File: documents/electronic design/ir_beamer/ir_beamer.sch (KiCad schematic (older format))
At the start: 10 parts, among them P1 STM32F103_header, U1 74HC595D

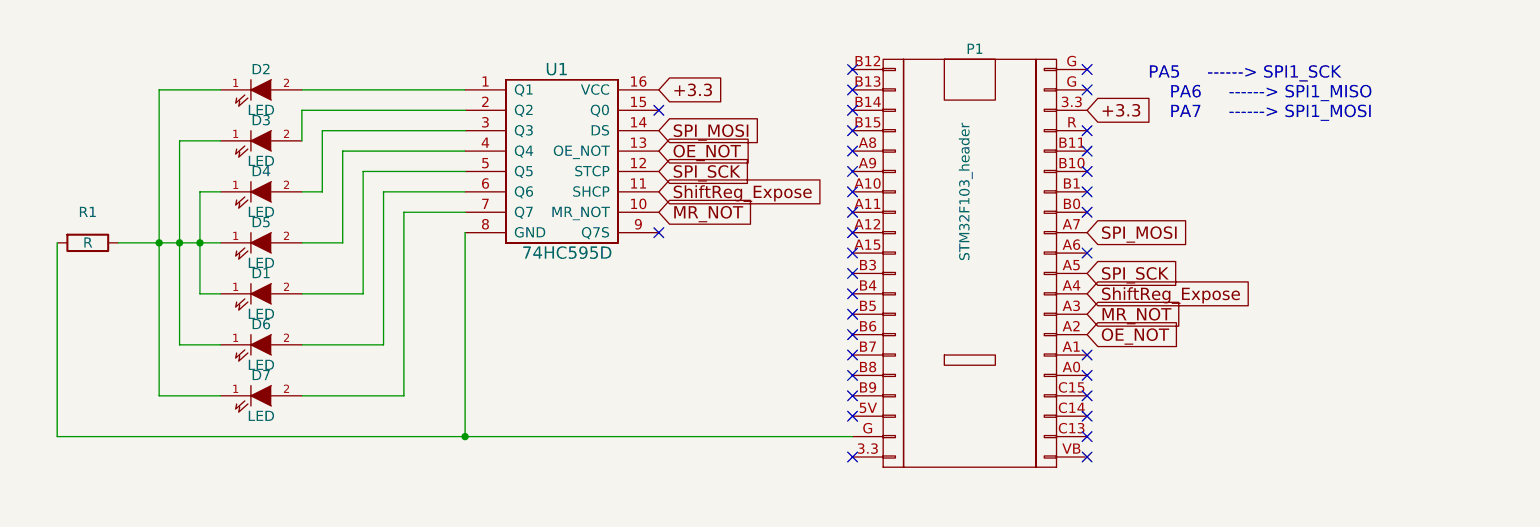
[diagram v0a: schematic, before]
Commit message: update pcb
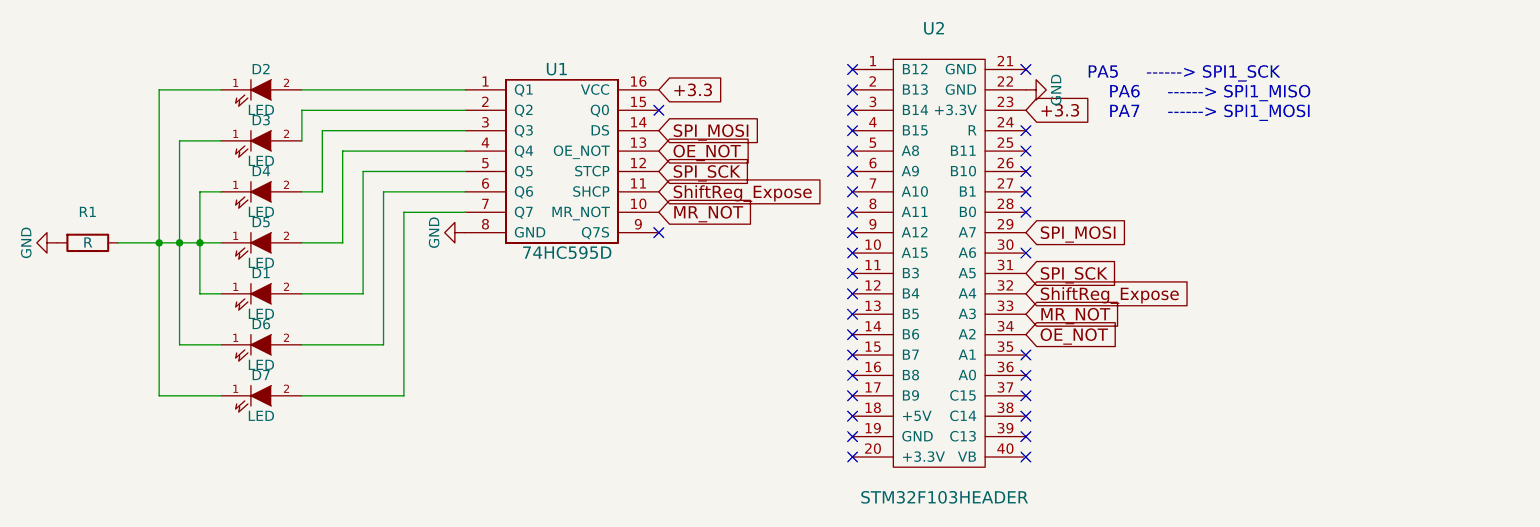
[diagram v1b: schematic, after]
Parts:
- removed P1: STM32F103_header, footprints:STM32F103C8T6_pin_header, symbol STM32F103_header
- added U2: STM32F103HEADER, symbol STM32F103HEADER
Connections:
- net +3.3: now also U2.23 (+3.3V)
- net MR_NOT: now also U2.33 (A3)
- net OE_NOT: now also U2.34 (A2)
- net SPI_MOSI: now also U2.29 (A7)
- net SPI_SCK: now also U2.31 (A5)
- net ShiftReg_Expose: now also U2.32 (A4)
- net GND: now reaches R1.2, U1.8 (GND)
- net GND: now also U2.22 (GND)
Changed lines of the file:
@@
 NoConn ~ 5300 3050
 NoConn ~ 5300 3150
-NoConn ~ 6450 3350
-NoConn ~ 6450 3250
-NoConn ~ 6450 3150
-NoConn ~ 6450 3050
-NoConn ~ 6450 2950
-NoConn ~ 6450 2850
-NoConn ~ 6450 2150
-NoConn ~ 6450 1950
-NoConn ~ 6450 1850
-NoConn ~ 6450 1750
+NoConn ~ 6150 3350
+NoConn ~ 6150 3250
+NoConn ~ 6150 3150
+NoConn ~ 6150 3050
+NoConn ~ 6150 2950
+NoConn ~ 6150 2850
+NoConn ~ 6150 2150
+NoConn ~ 6150 1950
+NoConn ~ 6150 1850
+NoConn ~ 6150 1750
 $Comp
 L LED D1
@@
 	1    0    0    -1
 $EndComp
-$Comp
-L STM32F103_header P1
-U 1 1 578765C4
-P 5500 2400
-F 0 "P1" H 5900 3450 50  0000 C CNN
-F 1 "STM32F103_header" V 5850 2750 50  0000 C CNN
-F 2 "footprints:STM32F103C8T6_pin_header" H 5500 2400 50  0001 C CNN
-F 3 "" H 5500 2400 50  0000 C CNN
-	1    5500 2400
-	1    0    0    -1
-$EndComp
-Text Notes 6750 1700 0    60   ~ 0
+Text Notes 6450 1700 0    60   ~ 0
     PA5     ------> SPI1_SCK\n    PA6     ------> SPI1_MISO\n    PA7     ------> SPI1_MOSI
-Text GLabel 6450 2450 2    60   Input ~ 0
+Text GLabel 6150 2450 2    60   Input ~ 0
 SPI_SCK
-Text GLabel 6450 2250 2    60   Input ~ 0
+Text GLabel 6150 2250 2    60   Input ~ 0
 SPI_MOSI
 Text GLabel 4350 1950 2    60   Input ~ 0
@@
 Text GLabel 4350 1750 2    60   Input ~ 0
 SPI_MOSI
-Text GLabel 6450 2550 2    60   Input ~ 0
+Text GLabel 6150 2550 2    60   Input ~ 0
 ShiftReg_Expose
 Text GLabel 4350 2050 2    60   Input ~ 0
 ShiftReg_Expose
-Text GLabel 6450 1650 2    60   Input ~ 0
+Text GLabel 6150 1650 2    60   Input ~ 0
 +3.3
 Text GLabel 4350 1550 2    60   Input ~ 0
@@
 NoConn ~ 4350 2250
 NoConn ~ 4350 1650
-Text GLabel 6450 2750 2    60   Input ~ 0
+Text GLabel 6150 2750 2    60   Input ~ 0
 OE_NOT
-Text GLabel 6450 2650 2    60   Input ~ 0
+Text GLabel 6150 2650 2    60   Input ~ 0
 MR_NOT
 Text GLabel 4350 1850 2    60   Input ~ 0
@@
 MR_NOT
 NoConn ~ 5300 1950
-NoConn ~ 6450 2350
+NoConn ~ 6150 2350
 NoConn ~ 5300 3350
-NoConn ~ 6450 1450
-NoConn ~ 6450 1550
 Wire Wire Line
 	2600 1550 3400 1550
@@
 Wire Wire Line
 	1900 3050 2200 3050
-NoConn ~ 6450 2050
-Wire Wire Line
-	1400 3250 5300 3250
-Wire Wire Line
-	3400 3250 3400 2250
-Wire Wire Line
-	1400 2300 1400 3250
-Connection ~ 3400 3250
+NoConn ~ 6150 2050
+$Comp
+L GND #PWR01
+U 1 1 5787B950
+P 1400 2300
+F 0 "#PWR01" H 1400 2050 50  0001 C CNN
+F 1 "GND" H 1400 2150 50  0000 C CNN
+F 2 "" H 1400 2300 50  0000 C CNN
+F 3 "" H 1400 2300 50  0000 C CNN
+	1    1400 2300
+	0    1    1    0
+$EndComp
+$Comp
+L STM32F103HEADER U2
+U 1 1 5787BBF4
+P 5550 2500
+F 0 "U2" H 5700 3750 60  0000 C CNN
+F 1 "STM32F103HEADER" H 5750 1450 60  0000 C CNN
+F 2 "" H 4900 3500 60  0000 C CNN
+F 3 "" H 4900 3500 60  0000 C CNN
+	1    5550 2500
+	1    0    0    -1
+$EndComp
+$Comp
+L GND #PWR02
+U 1 1 5787C121
+P 3400 2250
+F 0 "#PWR02" H 3400 2000 50  0001 C CNN
+F 1 "GND" H 3400 2100 50  0000 C CNN
+F 2 "" H 3400 2250 50  0000 C CNN
+F 3 "" H 3400 2250 50  0000 C CNN
+	1    3400 2250
+	0    1    1    0
+$EndComp
+$Comp
+L GND #PWR03
+U 1 1 5787C14A
+P 6150 1550
+F 0 "#PWR03" H 6150 1300 50  0001 C CNN
+F 1 "GND" H 6150 1400 50  0000 C CNN
+F 2 "" H 6150 1550 50  0000 C CNN
+F 3 "" H 6150 1550 50  0000 C CNN
+	1    6150 1550
+	0    -1   -1   0
+$EndComp
+NoConn ~ 6150 1450
+NoConn ~ 5300 3250
 $EndSCHEMATC
